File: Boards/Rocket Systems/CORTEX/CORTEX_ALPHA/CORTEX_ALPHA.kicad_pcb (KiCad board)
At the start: 2 copper layers, 135 x 92.5 mm, 6 parts, among them U1 NUCLEO-F302R8, U2 E28-2G4M27S_LoRa, U3 MAX485_MODULE_5V_LOGIC_TLL_TO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

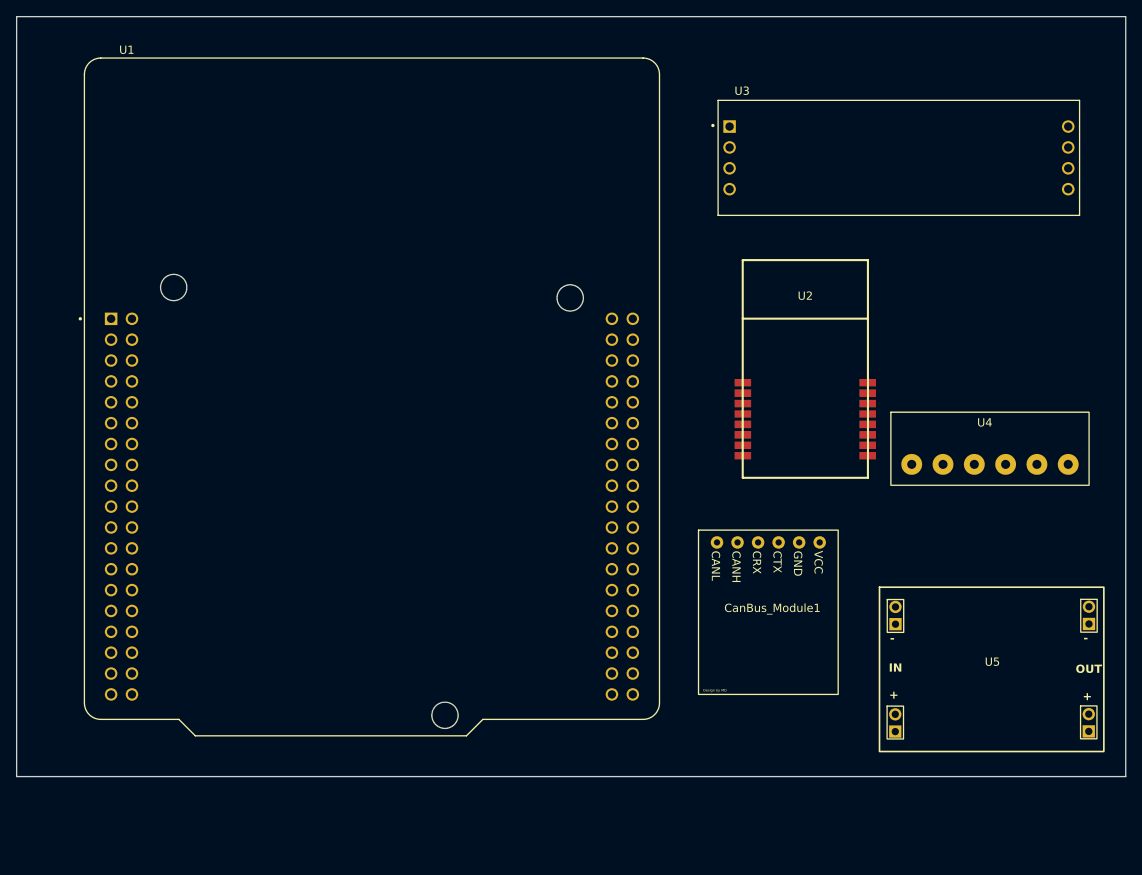
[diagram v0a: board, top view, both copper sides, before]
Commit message: Cortex Update
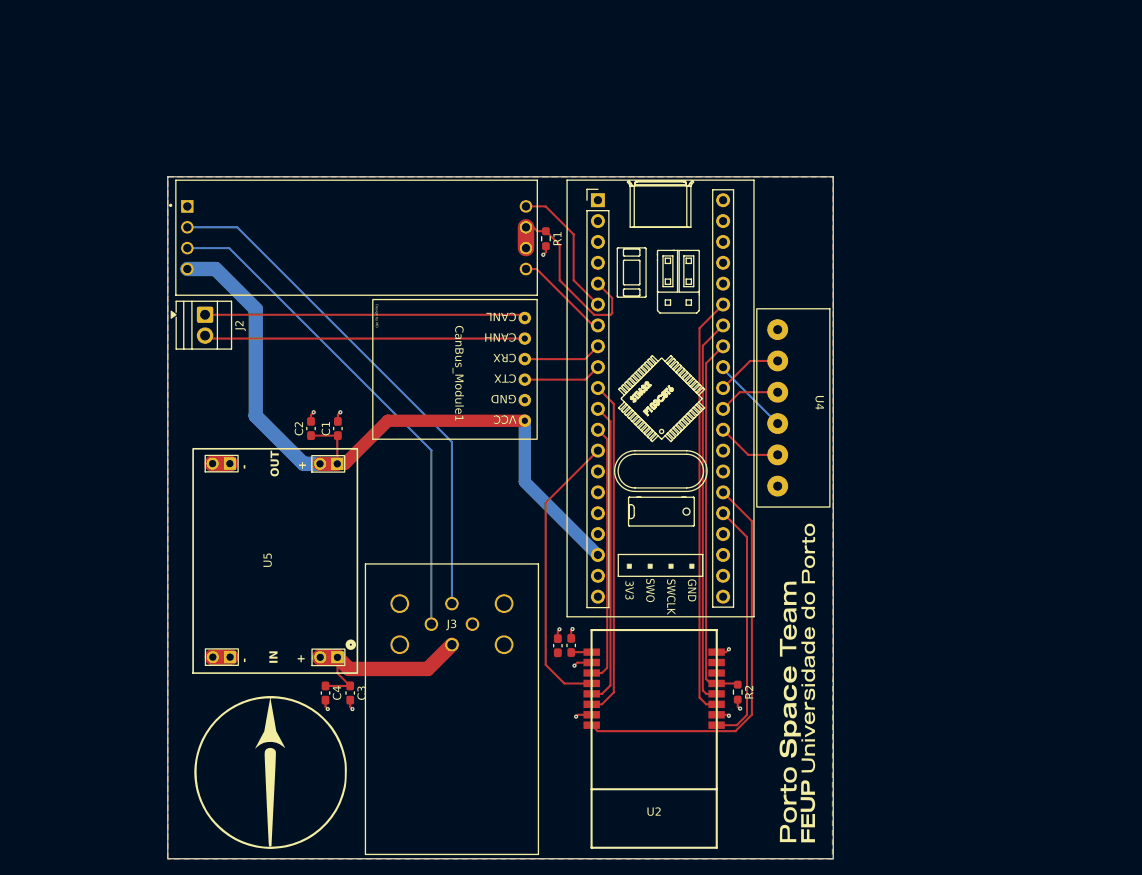
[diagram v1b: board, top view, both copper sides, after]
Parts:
- added C1: 10uF, Capacitor_SMD:C_0603_1608Metric_Pad1.08x0.95mm_HandSolder, F.Cu at (120.6, 89.1)
- added C2: 47uF, Capacitor_SMD:C_0603_1608Metric_Pad1.08x0.95mm_HandSolder, F.Cu at (117.3, 89.1)
- added C3: 47uF, Capacitor_SMD:C_0603_1608Metric_Pad1.08x0.95mm_HandSolder, F.Cu at (122.1, 121.3)
- added C4: 10uF, Capacitor_SMD:C_0603_1608Metric_Pad1.08x0.95mm_HandSolder, F.Cu at (119.1, 121.3)
- added C5: 100uF, Capacitor_SMD:C_0603_1608Metric_Pad1.08x0.95mm_HandSolder, F.Cu at (147.4, 115.6)
- added C6: 0.1uF, Capacitor_SMD:C_0603_1608Metric_Pad1.08x0.95mm_HandSolder, F.Cu at (149.0, 115.5)
- added G***: LOGO, FEUP-text:Feup-text, F.Cu at (176.6, 120.1)
- added G***: LOGO, LogoPST:LogoPST, F.Cu at (112.4, 131.0)
- added J2: Screw_Terminal_01x02, TerminalBlock:TerminalBlock_Xinya_XY308-2.54-2P_1x02_P2.54mm_Horizontal, F.Cu at (104.4, 75.3)
- added J3: 1200700164, CONN_1200700164_MOL:CONN_1200700164_MOL, F.Cu at (134.5, 115.4)
- added R1: 1K, Resistor_SMD:R_0603_1608Metric_Pad0.98x0.95mm_HandSolder, F.Cu at (145.9, 66.0)
- added R2: 10K, Resistor_SMD:R_0603_1608Metric_Pad0.98x0.95mm_HandSolder, F.Cu at (169.3, 121.2)
- U1: value NUCLEO-F302R8 -> YAAJ_BluePill; footprint MyLibrary:MODULE_NUCLEO-F302R8 -> STM32 Blue Pill:YAAJ_BluePill_1
- moved U5 88.6 mm to (112.6, 105.2), turned to 90 degrees
- moved U3 66.7 mm to (122.9, 65.9)
- moved CanBus_Module1 47.0 mm to (135.9, 82.4), turned to -90 degrees
- moved U2 37.6 mm to (159.1, 120.8), turned to 180 degrees
- moved U1 36.5 mm to (152.3, 61.3)
- moved U4 17.6 mm to (181.8, 86.0), turned to -90 degrees
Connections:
- CanBus_Module1 pad 1: unconnected-(CanBus_Module1-CANL-Pad1) -> Net-(CanBus_Module1-CANL)
- CanBus_Module1 pad 2: unconnected-(CanBus_Module1-CANH-Pad2) -> Net-(CanBus_Module1-CANH)
- CanBus_Module1 pad 3: unconnected-(CanBus_Module1-CRX-Pad3) -> /CAN_RX
- CanBus_Module1 pad 4: unconnected-(CanBus_Module1-CTX-Pad4) -> /CAN_TX
- CanBus_Module1 pad 5: unconnected-(CanBus_Module1-GND-Pad5) -> GND
- CanBus_Module1 pad 6: unconnected-(CanBus_Module1-VCC-Pad6) -> +5V
- U2 pad 1: unconnected-(U2-3.3V-Pad1) -> +3.3V
- U2 pad 10: unconnected-(U2-GND-Pad10) -> GND
- U2 pad 11: unconnected-(U2-NRESET-Pad11) -> /ANT_NRESET
- U2 pad 12: unconnected-(U2-BUSY-Pad12) -> /ANT_BUSY
- U2 pad 13: unconnected-(U2-DI01-Pad13) -> /ANT_DIO1
- U2 pad 16: unconnected-(U2-GND-Pad16) -> GND
- U2 pad 2: unconnected-(U2-GND-Pad2) -> GND
- U2 pad 3: unconnected-(U2-MISO_TX-Pad3) -> /ANT_MISO
- U2 pad 4: unconnected-(U2-MOSI_RX-Pad4) -> /ANT_MOSI
- U2 pad 5: unconnected-(U2-SCK_RTS-Pad5) -> /ANT_SCK
- U2 pad 6: unconnected-(U2-NSS_CTS-Pad6) -> /ANT_NSS
- U2 pad 7: unconnected-(U2-GND-Pad7) -> GND
- U2 pad 8: unconnected-(U2-RX_EN-Pad8) -> /ANT_RX_EN
- U2 pad 9: unconnected-(U2-TX_EN-Pad9) -> /ANT_TX_EN
- U3 pad 1: unconnected-(U3-GND-Pad1) -> GND
- U3 pad 2: unconnected-(U3-A-Pad2) -> /RS_A
- U3 pad 3: unconnected-(U3-B-Pad3) -> /RS_B
- U3 pad 4: unconnected-(U3-VCC-Pad4) -> +5V
- U3 pad 5: unconnected-(U3-RO-Pad5) -> /RS_RX
- U3 pad 6: unconnected-(U3-RE-Pad6) -> /RS_ENABLE
- U3 pad 7: unconnected-(U3-DE-Pad7) -> /RS_ENABLE
- U3 pad 8: unconnected-(U3-DI-Pad8) -> /RS_TX
- U4 pad 1: unconnected-(U4-GND-Pad1) -> GND
- U4 pad 2: unconnected-(U4-MISO-Pad2) -> /SD_MISO
- U4 pad 3: unconnected-(U4-CLK-Pad3) -> /SD_CLK
- U4 pad 4: unconnected-(U4-MOSI-Pad4) -> /SD_MOSI
- U4 pad 5: unconnected-(U4-CS-Pad5) -> /SD_CS
- U4 pad 6: unconnected-(U4-3.3V-Pad6) -> +3.3V
- U5 pad 1: unconnected-(U5-IN+-Pad1) -> /+12.8V
- U5 pad 2: unconnected-(U5-IN--Pad2) -> GND
- U5 pad 3: unconnected-(U5-OUT+-Pad3) -> +5V
- U5 pad 4: unconnected-(U5-OUT--Pad4) -> GND
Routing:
- net +5V: track 0.00 -> 87.5 mm
- net /RS_A: track 0.00 -> 62.7 mm
- net /RS_B: track 0.00 -> 61.1 mm
- net /ANT_NRESET: track 0.00 -> 51.4 mm
- net /ANT_RX_EN: track 0.00 -> 49.1 mm
- net /ANT_BUSY: track 0.00 -> 47.3 mm
- net /ANT_DIO1: track 0.00 -> 45.5 mm
- net /ANT_NSS: track 0.00 -> 41.1 mm
- net Net-(CanBus_Module1-CANL): track 0.00 -> 39.1 mm
- net Net-(CanBus_Module1-CANH): track 0.00 -> 39.1 mm
- net /ANT_SCK: track 0.00 -> 37.0 mm
- net /ANT_MOSI: track 0.00 -> 35.2 mm
- net /ANT_MISO: track 0.00 -> 31.6 mm
- net /ANT_TX_EN: track 0.00 -> 30.0 mm
- net /+12.8V: track 0.00 -> 25.0 mm
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- added copper zone on F.Cu, net +3.3V
- added copper zone on B.Cu, net GND
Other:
- board size 135 x 92.5 mm -> 81 x 83 mm
